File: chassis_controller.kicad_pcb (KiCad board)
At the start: 2 copper layers, 99.3 x 72.7 mm, 132 parts, among them J1 Screw_Terminal_01x02, J10 Conn_01x04_Pin, J12 Conn_01x04_Pin, J13 Conn_01x04_Pin, J14 Conn_01x04_Pin, J15 Conn_01x04_Pin, J16 Conn_01x04_Pin, J17 Conn_01x04_Pin, J18 Conn_01x03_Pin, J19 Conn_01x03_Pin, J2 Conn_01x04_Pin, J20 Conn_01x03_Pin, J21 Conn_01x04_Pin, J22 Conn_01x03_Pin, J23 Conn_01x03_Pin, J24 Conn_01x03_Pin, J25 Conn_01x03_Pin, J26 Conn_01x06_Pin, J3 Conn_01x02_Pin, J4 Conn_01x02_Pin, J5 Conn_01x03_Pin, J6 Conn_01x03_Pin, J7 Conn_01x04_Pin, J8 Conn_01x04_Pin, J9 Conn_01x04_Pin, Q1 NMOS, Q2 HSBA100P04, Q4 HSBA100P04, U1 AP64500SP-13, U2 AMS1117-3.3, U3 DSHP04TSGER, U4 STM32F407VGT6TR, U5 PCA9685PW,118, U6 PCA9685PW,118, U7 MPU-6050, U8 SN65HVD230DR, X1 X32258MOB4SI

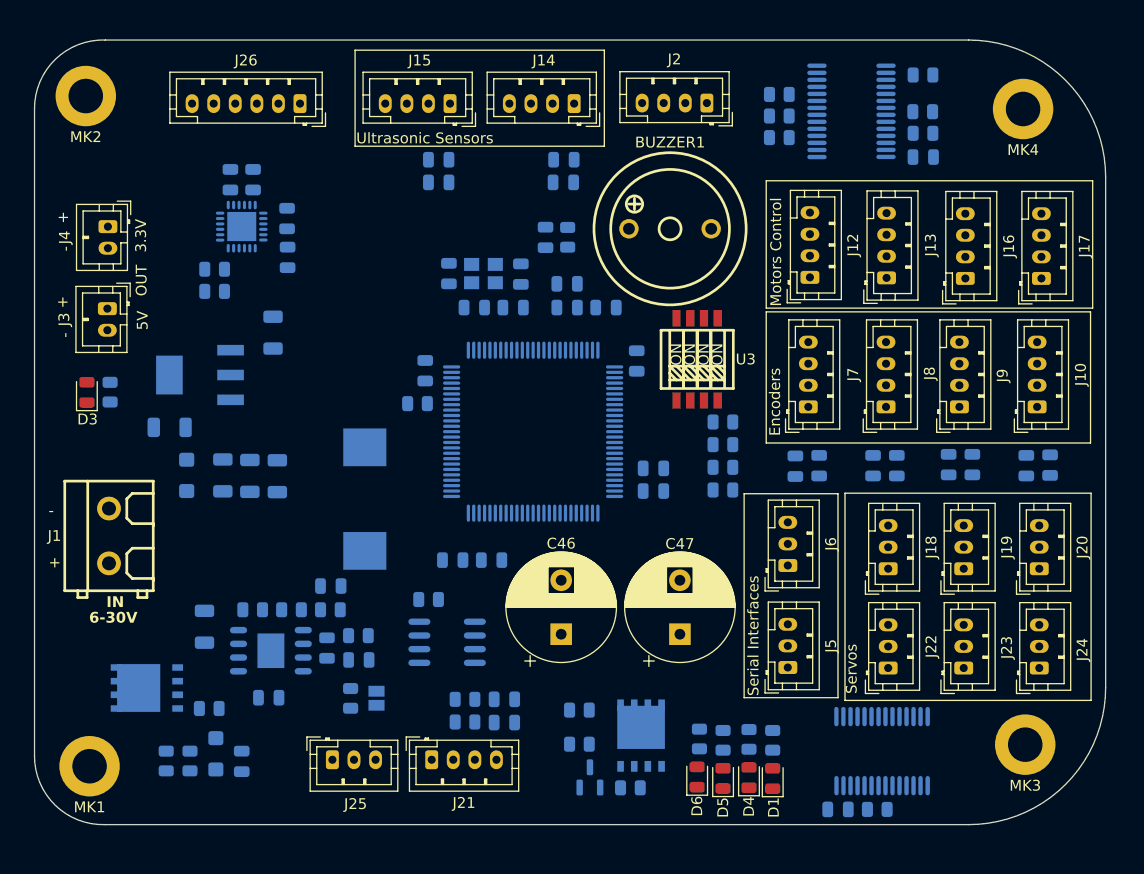
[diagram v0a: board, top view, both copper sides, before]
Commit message: Update project
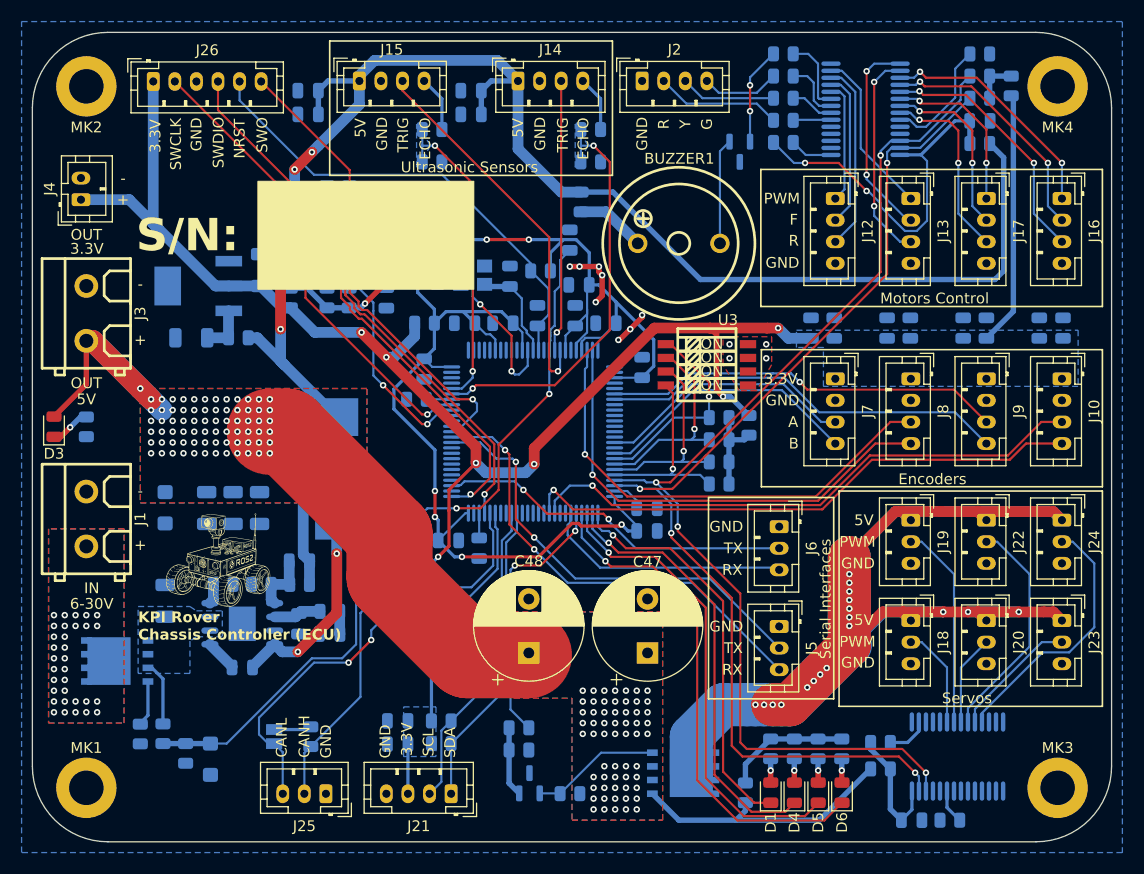
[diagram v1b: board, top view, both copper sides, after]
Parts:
- removed C39: 10nF, Capacitor_SMD:C_0805_2012Metric
- added C48: 1000uF, Capacitor_THT:CP_Radial_D10.0mm_P5.00mm, F.Cu at (150.0, 117.5)
- added G***: LOGO, kpi-rover:kpi-rover-logo, F.Cu at (121.3, 108.7)
- added Q3: NMOS, Package_TO_SOT_SMD:SOT-23, B.Cu at (169.6, 71.1)
- added R36: 4.7k, Resistor_SMD:R_0805_2012Metric, B.Cu at (173.6, 70.2)
- added R37: 4.7k, Resistor_SMD:R_0805_2012Metric, B.Cu at (182.6, 125.8)
- added R38: 0, Resistor_SMD:R_0805_2012Metric, B.Cu at (191.8, 70.3)
- added R39: 0, Resistor_SMD:R_0805_2012Metric, B.Cu at (182.6, 128.2)
- added R40: 0, Resistor_SMD:R_0805_2012Metric, B.Cu at (141.9, 118.4)
- added R41: 330, Resistor_SMD:R_0805_2012Metric, B.Cu at (173.6, 62.0)
- added R42: 1k, Resistor_SMD:R_0805_2012Metric, B.Cu at (155.7, 69.0)
- added R43: 1k, Resistor_SMD:R_0805_2012Metric, B.Cu at (141.0, 69.0)
- added R44: 2k, Resistor_SMD:R_0805_2012Metric, B.Cu at (155.7, 72.0)
- added R45: 2k, Resistor_SMD:R_0805_2012Metric, B.Cu at (141.0, 72.0)
- added R46: 0, Resistor_SMD:R_0805_2012Metric, B.Cu at (154.8, 75.7)
- added R47: 0, Resistor_SMD:R_0805_2012Metric, B.Cu at (123.1, 88.3)
- added R48: 0, Resistor_SMD:R_0805_2012Metric, B.Cu at (170.1, 130.5)
- added R49: 0, Resistor_SMD:R_0805_2012Metric, B.Cu at (127.9, 84.6)
- added R50: 0, Resistor_SMD:R_0805_2012Metric, B.Cu at (194.7, 65.0)
- added R51: 0, Resistor_SMD:R_0805_2012Metric, B.Cu at (170.4, 96.4)
- added R52: 0, Resistor_SMD:R_0805_2012Metric, B.Cu at (140.3, 87.0)
- C46: value 1000uF -> 100nF; footprint Capacitor_THT:CP_Radial_D10.0mm_P5.00mm -> Capacitor_SMD:C_0805_2012Metric; moved to B.Cu
- J3: value Conn_01x02_Pin -> Screw_Terminal_01x02; footprint Connector_JST:JST_PH_B2B-PH-K_1x02_P2.00mm_Vertical -> DB127V-5.08-2P-GN-S:CONN-TH_2P-P5.08
- moved C1 57.1 mm to (153.8, 79.2)
- moved C46 46.1 mm to (131.3, 75.2), turned to -90 degrees
- moved J22 16.4 mm to (192.4, 105.2), turned to -90 degrees
- moved J24 13.9 mm to (199.4, 105.2), turned to -90 degrees
- moved J26 13.8 mm to (115.2, 64.5), turned to 0 degrees
- moved C26 13.7 mm to (129.6, 65.4)
- moved C27 13.6 mm to (129.6, 67.6)
- moved D6 13.5 mm to (179.0, 130.4)
- moved C10 13.3 mm to (178.3, 87.4), turned to 90 degrees
- moved R11 13.2 mm to (179.0, 126.4)
- moved C12 13.2 mm to (185.3, 87.4), turned to 90 degrees
- moved C19 13.2 mm to (199.5, 87.4), turned to 90 degrees
- moved C17 13.1 mm to (192.4, 87.4), turned to 90 degrees
- moved C13 12.8 mm to (183.2, 87.4), turned to 90 degrees
- moved C11 12.8 mm to (176.2, 87.4), turned to 90 degrees
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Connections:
- BUZZER1 pad 1: +5V -> Net-(BUZZER1-Pad1)
- BUZZER1 pad 2: /BUZZER_OUT -> Net-(Q3-D)
- C15 pad 1: +5V -> Net-(U2-VIN)
- C36 pad 1: +5V -> Net-(U5-VDD)
- C37 pad 1: +5V -> Net-(U6-VDD)
- C43 pad 1: +3.3V -> Net-(U7-VDD)
- C46 pad 1: /SERVO_5V -> GND
- C46 pad 2: GND -> Net-(U7-VDD)
- C47 pad 1: /SERVO_5V -> +5V
- J14 pad 4: /USS1_ECHO -> Net-(J14-Pin_4)
- J15 pad 4: /USS2_ECHO -> Net-(J15-Pin_4)
- R1 pad 2: +5V -> Net-(R1-Pad2)
- R11 pad 2: +5V -> Net-(R1-Pad2)
- R22 pad 1: +3.3V -> Net-(R22-Pad1)
- R23 pad 1: +3.3V -> Net-(R22-Pad1)
- R24 pad 1: +3.3V -> Net-(R22-Pad1)
- R25 pad 1: +3.3V -> Net-(R22-Pad1)
- R28 pad 1: +5V -> Net-(R28-Pad1)
- R29 pad 1: +5V -> Net-(R28-Pad1)
- R30 pad 1: +3.3V -> Net-(U7-VDD)
- R31 pad 1: +3.3V -> Net-(U7-VDD)
- R4 pad 2: +5V -> Net-(R1-Pad2)
- R7 pad 2: +5V -> Net-(R1-Pad2)
- U2 pad 3: +5V -> Net-(U2-VIN)
- U5 pad 1: GND -> Net-(U5-A0)
- U5 pad 28: +5V -> Net-(U5-VDD)
- U6 pad 2: GND -> Net-(U6-A1)
- U6 pad 28: +5V -> Net-(U6-VDD)
- U7 pad 13: +3.3V -> Net-(U7-VDD)
- U7 pad 8: +3.3V -> Net-(U7-VDD)
- U7 pad 9: unconnected-(U7-AD0-Pad9) -> GND
- U8 pad 3: +3.3V -> Net-(U8-VCC)
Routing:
- net +3.3V: track 0.00 -> 302.1 mm, vias 0 -> 13
- net +5V: track 0.00 -> 241.8 mm, vias 0 -> 136
- net /SERVO_5V: track 0.00 -> 135.8 mm, vias 0 -> 18
- net /PCA_I2C_SCL: track 0.00 -> 103.3 mm, vias 0 -> 4
- net /PCA_I2C_SDA: track 0.00 -> 102.7 mm, vias 0 -> 4
- net /POWER_SUPPLY_ADC: track 0.00 -> 69.3 mm, vias 0 -> 2
- net /SWCLK: track 0.00 -> 53.3 mm, vias 0 -> 1
- net /ENC4_B: track 0.00 -> 52.7 mm, vias 0 -> 1
- net /ENC4_A: track 0.00 -> 52.7 mm, vias 0 -> 1
- net /SWDIO: track 0.00 -> 51.2 mm, vias 0 -> 1
- net /STATUS_LED_4: track 0.00 -> 47.1 mm, vias 0 -> 1
- net /ENC2_A: track 0.00 -> 44.4 mm, vias 0 -> 1
- net /ENC2_B: track 0.00 -> 44.2 mm, vias 0 -> 1
- net /NRST: track 0.00 -> 44.2 mm
- net /STATUS_LED_3: track 0.00 -> 43.9 mm, vias 0 -> 1
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- added copper zone on B.Cu, net +3.3V
- added copper zone on B.Cu, net +5V
- added copper zone on F.Cu, net +5V
- added copper zone on B.Cu, net /USS1_ECHO
- added copper zone on B.Cu, net /USS2_ECHO
- added copper zone on B.Cu, net GND
- added copper zone on F.Cu, net GND
- added copper zone on B.Cu, net Net-(U1-EN)
- added copper zone on B.Cu, net VCC
- added copper zone on F.Cu, net VCC
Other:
- board size 99.3 x 72.7 mm -> 100 x 75 mm
- board text added: "A"
- board text added: "B"
- board text added: "CANH"
- board text added: "CANL"
- board text added: "ECHO"
- board text added: "F"
- board text added: "G"
- board text added: "GND"
- board text added: "KPI Rover Chassis Controller (ECU)"
- board text added: "NRST"
- board text added: "PWM"
- board text added: "R"
- board text added: "RX"
- board text added: "S/N:"
- board text added: "SCL"
- board text added: "SDA"
- board text added: "SWCLK"
- board text added: "SWDIO"
- board text added: "SWO"
- board text added: "TRIG"
- board text added: "TX"
- board text added: "Y"
